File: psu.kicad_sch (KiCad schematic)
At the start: 13 parts, among them J13 Barrel_Jack_MountingPin, J14 Conn_02x01

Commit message: Replace Fuse with SMD part
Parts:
- F1: footprint Capacitor_THT:C_Rect_L7.0mm_W3.5mm_P5.00mm -> Fuse:Fuse_1812_4532Metric; Supplier https://www.digikey.ch/de/products/detail/bel-fuse-inc/0ZRP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 -> https://www.digikey.ch/de/products/detail/littelfuse-inc/18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
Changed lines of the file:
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@@
       (effects (font (size 1.27 1.27)))
     )
-    (property "Footprint" "Capacitor_THT:C_Rect_L7.0mm_W3.5mm_P5.00mm" (at 71.12 39.37 0)
+    (property "Footprint" "Fuse:Fuse_1812_4532Metric" (at 71.12 39.37 0)
       (effects (font (size 1.27 1.27)) (justify left) hide)
     )
-    (property "Datasheet" "https://www.onsemi.com/pdf/datasheet/1n5400-d.pdf" (at 66.04 40.64 0)
+    (property "Datasheet" "https://www.littelfuse.com/~/media/electronics/datasheets/resettable_ptcs/littelfuse_ptc_1812l_datasheet.pdf.pdf" (at 66.04 40.64 0)
       (effects (font (size 1.27 1.27)) hide)
     )
-    (property "Supplier" "https://www.digikey.ch/de/products/detail/bel-fuse-inc/0ZRP0090FF1E/9468255" (at 66.04 40.64 90)
+    (property "Supplier" "https://www.digikey.ch/de/products/detail/littelfuse-inc/1812L150-24MR/2023969" (at 66.04 40.64 90)
       (effects (font (size 1.27 1.27)) hide)
     )

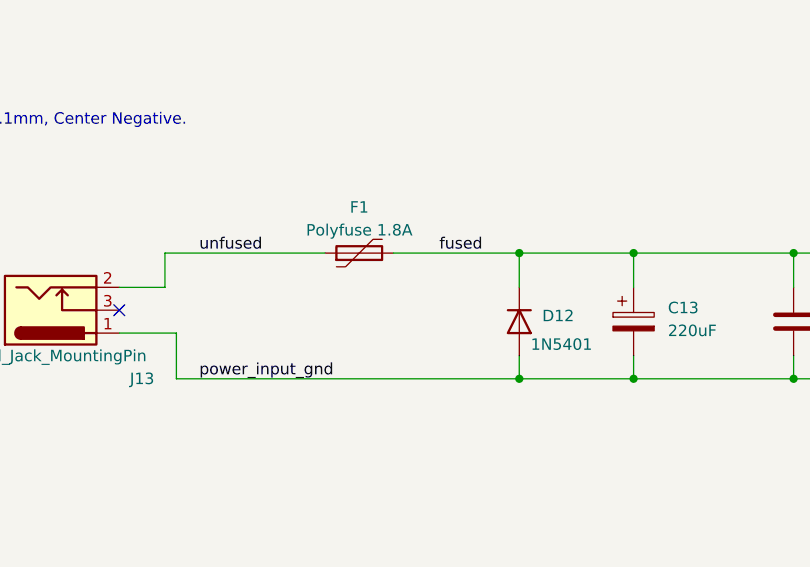
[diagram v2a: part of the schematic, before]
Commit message: Replace reverse power diode with MOSFET
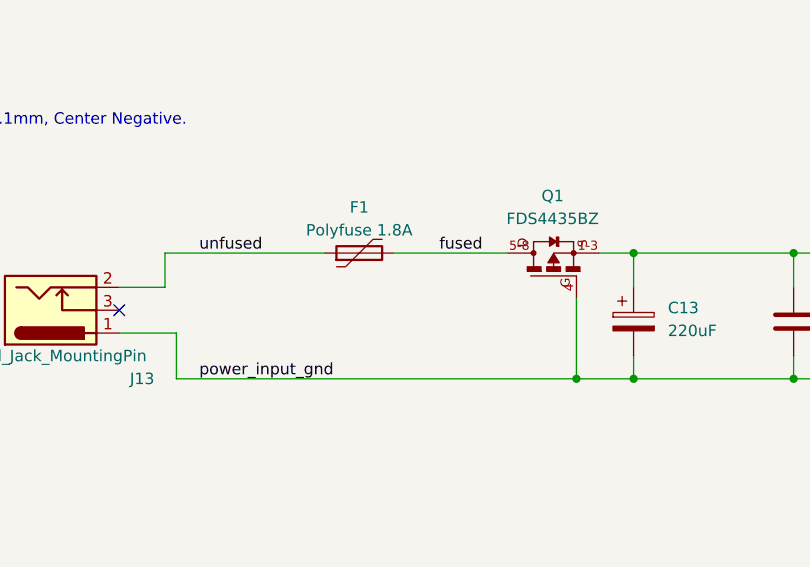
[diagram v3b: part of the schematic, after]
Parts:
- removed D12: 1N5401, Diode_THT:D_DO-201AD_P15.24mm_Horizontal, symbol Diode:1N5401
- added Q1: FDS4435BZ, Pedalboard Library:SO08-E3, symbol FDS4435BZ:FDS4435BZ
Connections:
- net fused: now also Q1.5-8; no longer C13.1, C16.1, L6.1
- net power_input_gnd: now also Q1.4
- new net: C13.1, C16.1, L6.1, Q1.1-3
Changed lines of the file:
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@@
   (junction (at 227.33 53.34) (diameter 0) (color 0 0 0 0)
   )
+  (junction (at 96.52 40.64) (diameter 0) (color 0 0 0 0)
+  )
+  (junction (at 90.17 54.61) (diameter 0) (color 0 0 0 0)
+  )
   (junction (at 154.94 54.61) (diameter 0) (color 0 0 0 0)
   )
   (junction (at 227.33 22.86) (diameter 0) (color 0 0 0 0)
   )
-  (junction (at 83.82 40.64) (diameter 0) (color 0 0 0 0)
-  )
   (junction (at 137.16 40.64) (diameter 0) (color 0 0 0 0)
   )
@@
   (junction (at 114.3 40.64) (diameter 0) (color 0 0 0 0)
   )
-  (junction (at 96.52 40.64) (diameter 0) (color 0 0 0 0)
-  )
   (junction (at 154.94 40.64) (diameter 0) (color 0 0 0 0)
-  )
-  (junction (at 83.82 54.61) (diameter 0) (color 0 0 0 0)
   )
   (junction (at 227.33 43.18) (diameter 0) (color 0 0 0 0)
@@
   (no_connect (at 39.37 46.99))
   (no_connect (at 212.09 48.26))
+  (wire (pts (xy 90.17 54.61) (xy 96.52 54.61))
+    (stroke (width 0) (type default))
+  )
   (wire (pts (xy 234.95 73.66) (xy 234.95 76.2))
     (stroke (width 0) (type default))
@@
     (stroke (width 0) (type default))
   )
+  (wire (pts (xy 90.17 45.72) (xy 90.17 54.61))
+    (stroke (width 0) (type default))
+  )
   (wire (pts (xy 137.16 27.94) (xy 137.16 22.86))
     (stroke (width 0) (type default))
@@
     (stroke (width 0) (type default))
   )
+  (wire (pts (xy 92.71 40.64) (xy 96.52 40.64))
+    (stroke (width 0) (type default))
+  )
   (wire (pts (xy 227.33 22.86) (xy 227.33 43.18))
     (stroke (width 0) (type default))
@@
     (stroke (width 0) (type default))
   )
-  (wire (pts (xy 83.82 40.64) (xy 96.52 40.64))
-    (stroke (width 0) (type default))
-  )
   (wire (pts (xy 179.07 40.64) (xy 181.61 43.18))
     (stroke (width 0) (type default))
@@
     (stroke (width 0) (type default))
   )
-  (wire (pts (xy 83.82 40.64) (xy 83.82 44.45))
-    (stroke (width 0) (type default))
-  )
   (wire (pts (xy 137.16 73.66) (xy 227.33 73.66))
     (stroke (width 0) (type default))
@@
     (stroke (width 0) (type default))
   )
-  (wire (pts (xy 69.85 40.64) (xy 83.82 40.64))
+  (wire (pts (xy 69.85 40.64) (xy 82.55 40.64))
     (stroke (width 0) (type default))
   )
@@
     (stroke (width 0) (type default))
   )
-  (wire (pts (xy 83.82 54.61) (xy 96.52 54.61))
+  (wire (pts (xy 45.72 54.61) (xy 90.17 54.61))
     (stroke (width 0) (type default))
   )
@@
     (stroke (width 0) (type default))
   )
-  (wire (pts (xy 45.72 54.61) (xy 83.82 54.61))
-    (stroke (width 0) (type default))
-  )
   (wire (pts (xy 154.94 52.07) (xy 154.94 54.61))
-    (stroke (width 0) (type default))
-  )
-  (wire (pts (xy 83.82 52.07) (xy 83.82 54.61))
     (stroke (width 0) (type default))
   )
@@
   (label "vo" (at 195.58 22.86 0) (fields_autoplaced)
     (effects (font (size 1.27 1.27)) (justify left bottom))
-  )
-  (symbol (lib_id "Diode:1N5401") (at 83.82 48.26 270) (unit 1)
-    (in_bom yes) (on_board yes) (dnp no)
-    (property "Reference" "D12" (at 86.36 47.625 90)
-      (effects (font (size 1.27 1.27)) (justify left))
-    )
-    (property "Value" "1N5401" (at 85.09 50.8 90)
-      (effects (font (size 1.27 1.27)) (justify left))
-    )
-    (property "Footprint" "Diode_THT:D_DO-201AD_P15.24mm_Horizontal" (at 79.375 48.26 0)
-      (effects (font (size 1.27 1.27)) hide)
-    )
-    (property "Datasheet" "http://www.vishay.com/docs/88516/1n5400.pdf" (at 83.82 48.26 0)
-      (effects (font (size 1.27 1.27)) hide)
-    )
-    (property "Supplier" "https://www.digikey.ch/de/products/detail/onsemi/1N5401G/1485525" (at 83.82 48.26 0)
-      (effects (font (size 1.27 1.27)) hide)
-    )
-    (pin "1")
-    (pin "2")
-    (instances
-      (project "pedalboard-hw"
-        (path "/df521c2a-9827-4355-b809-366f4b88d5d7/0d7c87b0-1309-475f-a9d7-edcf3dee5e4e"
-          (reference "D12") (unit 1)
-        )
-      )
-    )
   )
   (symbol (lib_id "Device:C") (at 114.3 48.26 0) (unit 1)
@@
         )
       )
+    )
+  )
+  (symbol (lib_id "FDS4435BZ:FDS4435BZ") (at 87.63 40.64 90) (unit 1)
+    (in_bom yes) (on_board yes) (dnp no) (fields_autoplaced)
+    (property "Reference" "Q1" (at 87.5247 34.29 90)
+      (effects (font (size 1.27 1.27)))
+    )
+    (property "Value" "FDS4435BZ" (at 87.5247 36.83 90)
+      (effects (font (size 1.27 1.27)))
+    )
+    (property "Footprint" "Pedalboard Library:SO08-E3" (at 87.63 40.64 0)
+      (effects (font (size 1.27 1.27)) (justify bottom) hide)
+    )
+    (property "Datasheet" "" (at 87.63 40.64 0)
+      (effects (font (size 1.27 1.27)) hide)
+    )
+    (property "MF" "onsemi" (at 87.63 40.64 0)
+      (effects (font (size 1.27 1.27)) (justify bottom) hide)
+    )
+    (property "Package" "None" (at 87.63 40.64 0)
+      (effects (font (size 1.27 1.27)) (justify bottom) hide)
+    )
+    (property "MP" "FDS4435BZ" (at 87.63 40.64 0)
+      (effects (font (size 1.27 1.27)) (justify bottom) hide)
+    )
+    (pin "1-3")
+    (pin "4")
+    (pin "5-8")
+    (instances
+      (project "pedalboard-hw"
+        (path "/df521c2a-9827-4355-b809-366f4b88d5d7/0d7c87b0-1309-475f-a9d7-edcf3dee5e4e"
+          (reference "Q1") (unit 1)
+        )
+      )
